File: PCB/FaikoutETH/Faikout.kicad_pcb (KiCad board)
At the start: 2 copper layers, 70 x 70 mm, 73 parts, among them J1 1x5, J2 TC2030-USB-NL, J3 Reset, J4 RJ45_LED, Q1 BSS138PS, U1 KSZ8851SNL, U4 ESP32-S3-MINI-1, U5 TPS62933, Y1 Crystal_GND24

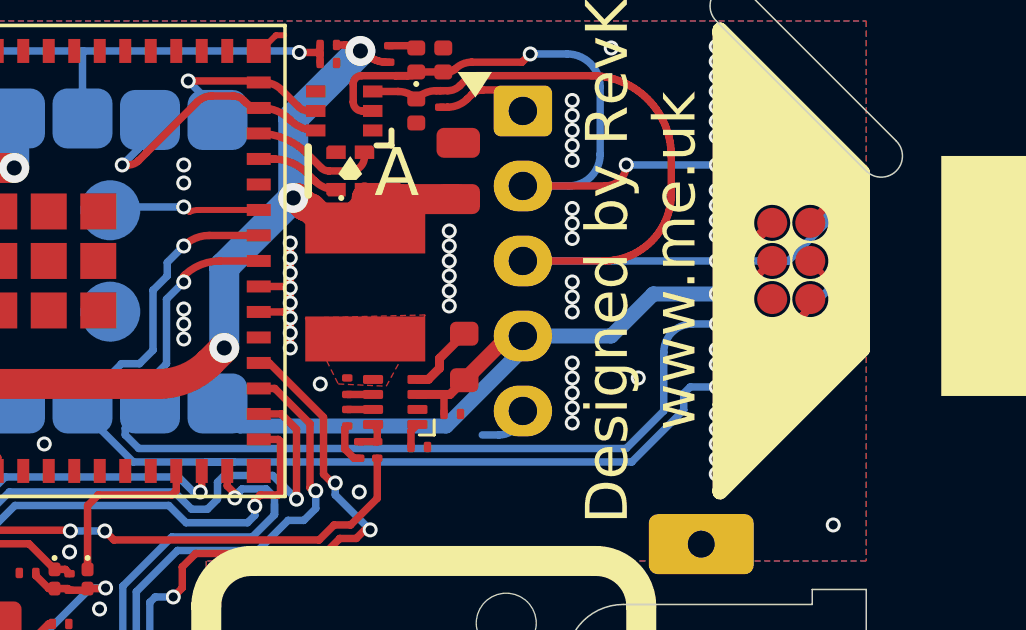
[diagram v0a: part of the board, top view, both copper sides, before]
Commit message: As ordered
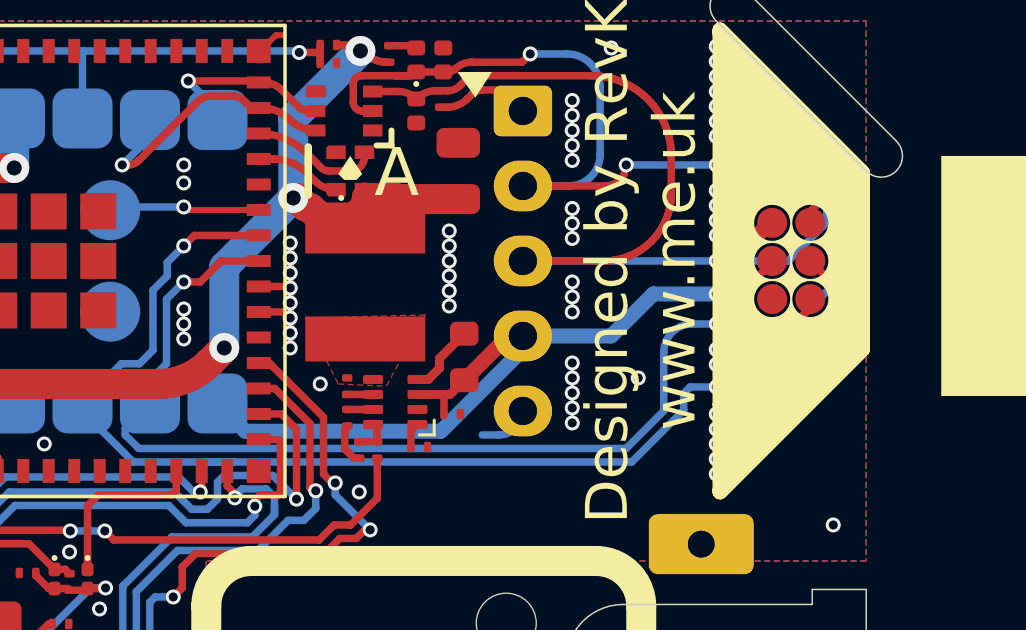
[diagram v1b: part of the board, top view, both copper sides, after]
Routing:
- net D+: track 42.1 -> 42.6 mm
